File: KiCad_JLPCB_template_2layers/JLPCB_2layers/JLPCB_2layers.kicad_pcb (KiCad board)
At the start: 2 copper layers, 119.9 x 95.2 mm, 64 parts, among them J1 Conn_02x08_Odd_Even, J2 Conn_02x08_Odd_Even, J3 Conn_02x05_Odd_Even, SW1 RST, SW2 OVR, SW3 SW_SPDT, U1 SM420561N, U2 SM420561N, U3 LM1117DT-3.3

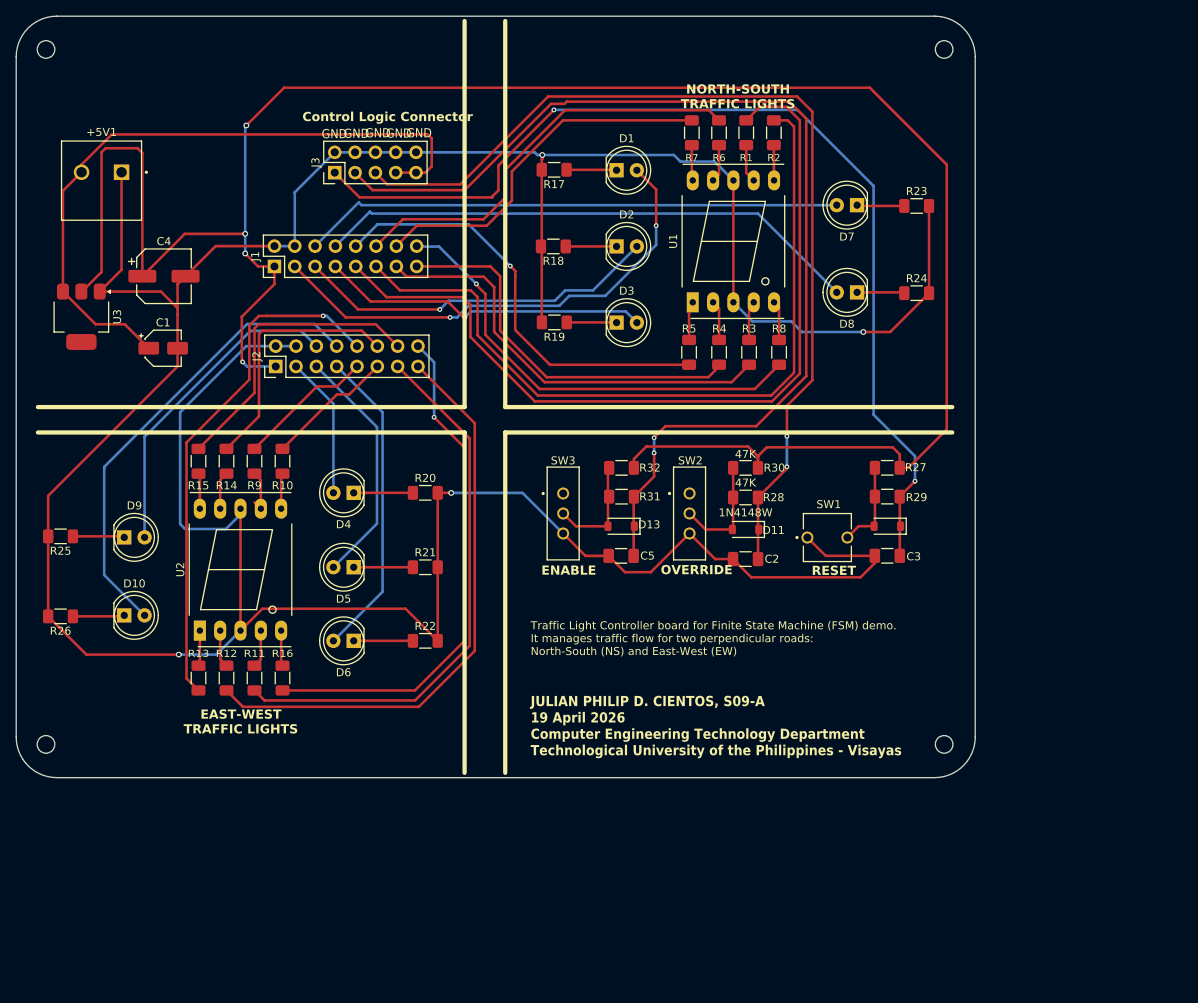
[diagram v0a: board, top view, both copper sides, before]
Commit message: Conversion of file to 10.0 to 9.0
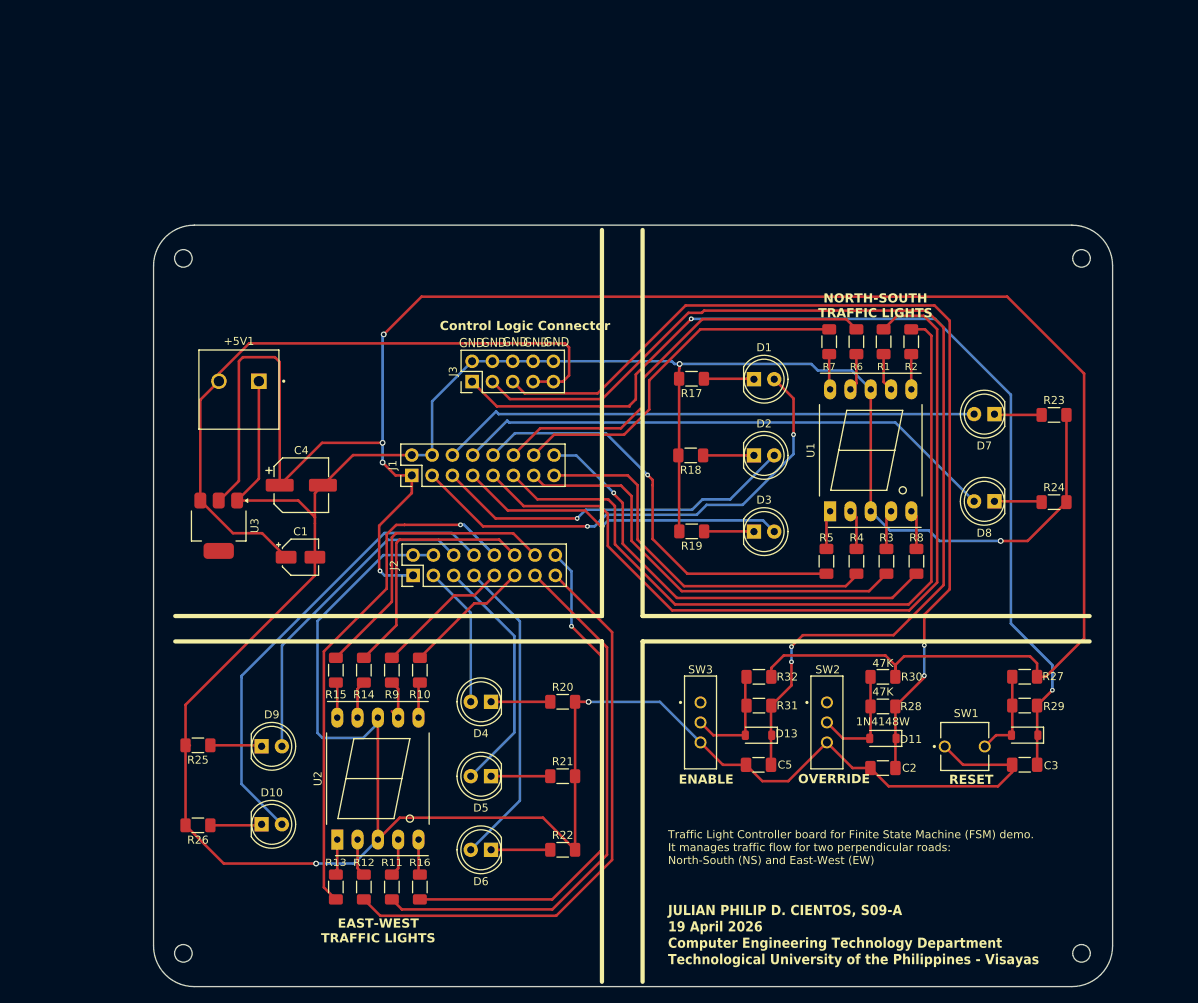
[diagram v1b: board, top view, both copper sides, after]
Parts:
- moved C3 31.3 mm to (156.4, 113.3)
- moved D12 31.3 mm to (156.4, 109.6)
- moved D8 31.3 mm to (152.6, 80.4)
- moved R1 31.3 mm to (138.7, 60.4)
- moved R27 31.3 mm to (156.4, 102.3)
- moved R29 31.3 mm to (156.4, 105.9)
- moved SW1 31.3 mm to (148.9, 111.0)
- moved U1 31.3 mm to (132.1, 81.6)
- moved C2 31.3 mm to (138.7, 113.7)
- moved D10 31.3 mm to (61.0, 120.7)
- moved D11 31.3 mm to (138.7, 110.0)
- moved D2 31.3 mm to (122.5, 74.6)
- moved D4 31.3 mm to (89.7, 105.4)
- moved D5 31.3 mm to (89.7, 114.7)
- moved D6 31.3 mm to (89.7, 123.9)
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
